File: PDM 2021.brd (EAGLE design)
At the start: 82.5 x 101.6 mm, 32 parts, among them K1 SR4M4012, Q1 SI7336ADP-T1-GE3

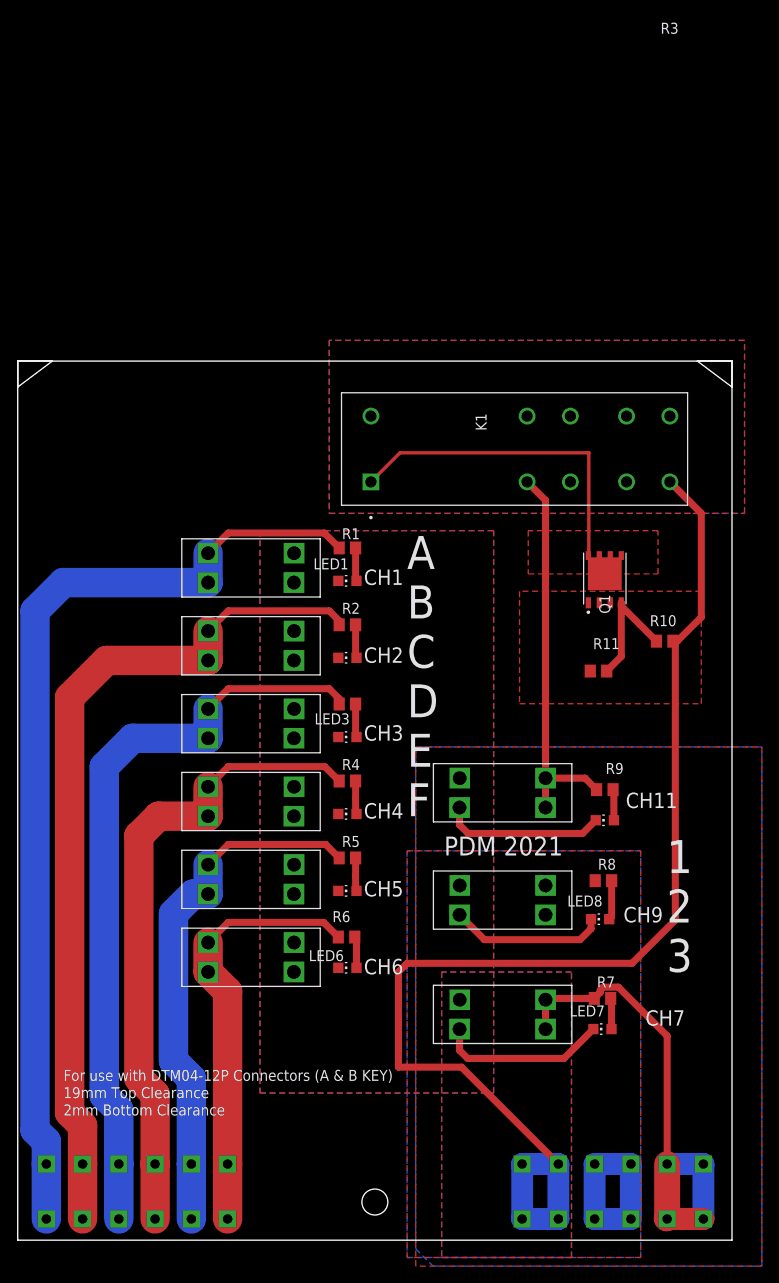
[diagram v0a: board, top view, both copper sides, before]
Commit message: Add files via upload
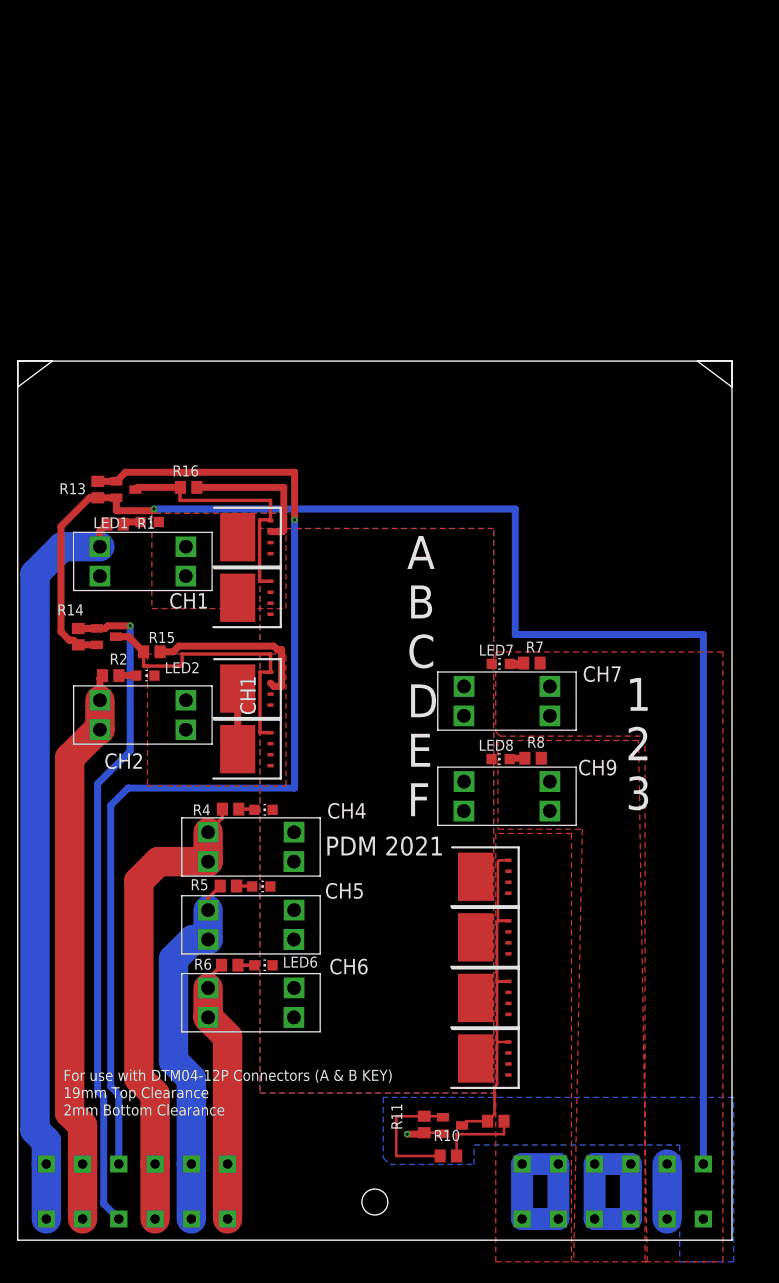
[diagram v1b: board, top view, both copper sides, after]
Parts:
- removed CH11, CH3: 3568FUSEHOLDER, ACC-MB-R0:3568
- removed K1: SR4M4012, SR4M4012:RELAY_SR4M4012
- removed LED3, LED9: (no value), led:CHIP-LED0805
- removed Q1: SI7336ADP-T1-GE3, SI7336ADP-T1-GE3:SI7141DPT1GE3
- removed R3, R9: (no value), rcl:R0805
- added R12, R13, R14, R15, R16: (no value), rcl:R0805
- added U$1, U$10, U$2, U$3, U$5, U$7, U$8, U$9: _CUSTOM_111_CUSTOM_SQJ407EP-T1_GE3, ACC-MB-R0:_CUSTOM_111_CUSTOM_TRANS_SIRA90DP-T1-GE3
- added U$11, U$12, U$6: RK7002BMT116, ACC-MB-R0:SOT23
- moved R10 64.5 mm to (49.8, 9.73)
- moved R11 56.1 mm to (47.0, 13.4), turned to 90 degrees
- moved LED7 43.8 mm to (55.8, 66.6)
- moved R7 39.6 mm to (59.4, 66.7), turned to 180 degrees
- moved CH7 36.2 mm to (61.5, 64.0)
- moved R2 28.0 mm to (10.8, 65.2)
- moved R1 27.0 mm to (11.2, 82.8)
- moved LED1 23.8 mm to (15.2, 83.0), turned to 270 degrees
- moved LED2 23.4 mm to (14.8, 65.2), turned to 270 degrees
- moved LED8 21.8 mm to (55.8, 55.6)
- moved R8 16.3 mm to (59.6, 55.7), turned to 180 degrees
- moved CH2 14.8 mm to (9.50, 59.0)
- moved R5 14.1 mm to (24.4, 40.9)
- moved R4 13.9 mm to (24.6, 49.8)
- moved R6 13.9 mm to (24.5, 31.8)
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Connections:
- removed net CH1: CH1.L1, CH1.L2, R1.1, U$4.6B, U$4.7B
- removed net CH3: CH3.L1, CH3.L2, R3.1, U$4.4B, U$4.9B
- removed net COMMON: CH1.R1, CH1.R2, CH11.R1, CH11.R2, CH2.R1, CH2.R2, CH3.R1, CH3.R2, CH4.R1, CH4.R2, CH5.R1, CH5.R2, CH6.R1, CH6.R2, CH7.R1, CH7.R2, CH9.R1, CH9.R2, LED1.C, LED2.C, LED3.C, LED4.C, LED5.C, LED6.C, LED7.C, LED8.C, LED9.C
- removed net N$12: K1.A1, Q1.5, Q1.6, Q1.7, Q1.8
- new net N$10: R10.1, R11.2, U$6.1
- new net N$13: R16.2, U$11.3, U$7.4, U$8.4
- new net N$16: R10.2, R12.2, U$1.1, U$1.2, U$1.3, U$2.1, U$2.2, U$2.3, U$3.1, U$3.2, U$3.3, U$4.11A, U$4.12A, U$4.1A, U$4.2A, U$5.1, U$5.2, U$5.3
- new net N$17: R15.2, U$10.4, U$12.3, U$9.4
- new net N$19: R14.2, U$12.1, U$4.4B
- new net N$9: CH1.R1, LED1.C, U$7.5, U$8.5
- net CH11: now also CH2.R1, CH2.R2, LED2.C, U$10.5, U$9.5; no longer K1.23, K1.33, K1.43, K1.A2, R10.2, U$4.11A, U$4.12A, U$4.1A, U$4.2A
- net CH8: no longer U$4.6A, U$4.7A
- net GND: now also R13.1, R14.1, U$11.2, U$12.2, U$4.6A, U$4.7A, U$6.2; no longer Q1.1, Q1.2, Q1.3
- net N$1: now also CH4.R1, CH4.R2, CH5.R1, CH5.R2, CH6.R1, CH6.R2, CH7.R1, CH7.R2, CH9.R1, CH9.R2, LED4.C, LED5.C, LED6.C, LED7.C, LED8.C, R15.1, R16.1, U$1.5, U$10.1, U$10.2, U$10.3, U$2.5, U$3.5, U$5.5, U$7.1, U$7.2, U$7.3, U$8.1, U$8.2, U$8.3, U$9.1, U$9.2, U$9.3; no longer LED9.A, R9.2
- net N$11: now also R12.1, U$1.4, U$2.4, U$3.4, U$5.4, U$6.3; no longer Q1.4, R10.1, R11.2
- net N$14: now also R13.2, U$11.1, U$4.9B; no longer CH11.L1, CH11.L2, K1.24, K1.34, K1.44, R9.1
- net N$7: now also CH1.L1, R1.1, U$4.6B, U$4.7B; no longer LED3.A, R3.2
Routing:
- net GND: track 0.00 -> 174.1 mm, vias 0 -> 2
- net CH11: track 143.6 -> 7.00 mm
- net CH1: track 112.4 -> 0.00 mm
- net CH3: track 86.9 -> 0.00 mm
- net N$7: track 3.85 -> 86.8 mm
- net N$14: track 45.3 -> 123.6 mm, vias 0 -> 1
- net N$19: track 0.00 -> 77.3 mm, vias 0 -> 1
- net CH8: track 67.0 -> 6.35 mm
- net COMMON: track 56.5 -> 0.00 mm
- net N$12: track 38.3 -> 0.00 mm
- net CH2: track 99.1 -> 65.1 mm
- net N$1: track 3.58 -> 36.8 mm
- net N$17: track 0.00 -> 33.2 mm
- net N$16: track 0.00 -> 30.6 mm
- net N$13: track 0.00 -> 29.3 mm
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- added copper zone on layer 16, net GND
- added copper zone on layer 1, net N$1
- added copper zone on layer 16, net N$1
- added copper zone on layer 1, net N$16
- added copper zone on layer 1, net N$9
- removed copper zone on layer 16, net CH10
- removed copper zone on layer 16, net CH11
- removed copper zone on layer 16, net CH8
- removed copper zone on layer 1, net COMMON
- removed copper zone on layer 16, net COMMON
- removed copper zone on layer 1, net GND
- removed copper zone on layer 1, net N$12
- removed copper zone on layer 16, net N$14
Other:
- board text removed: "CH11"
- board text removed: "CH3"
